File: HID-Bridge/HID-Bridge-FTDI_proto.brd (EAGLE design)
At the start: 33 x 20.3 mm, 7 parts, among them U1 FT232RLSSOP

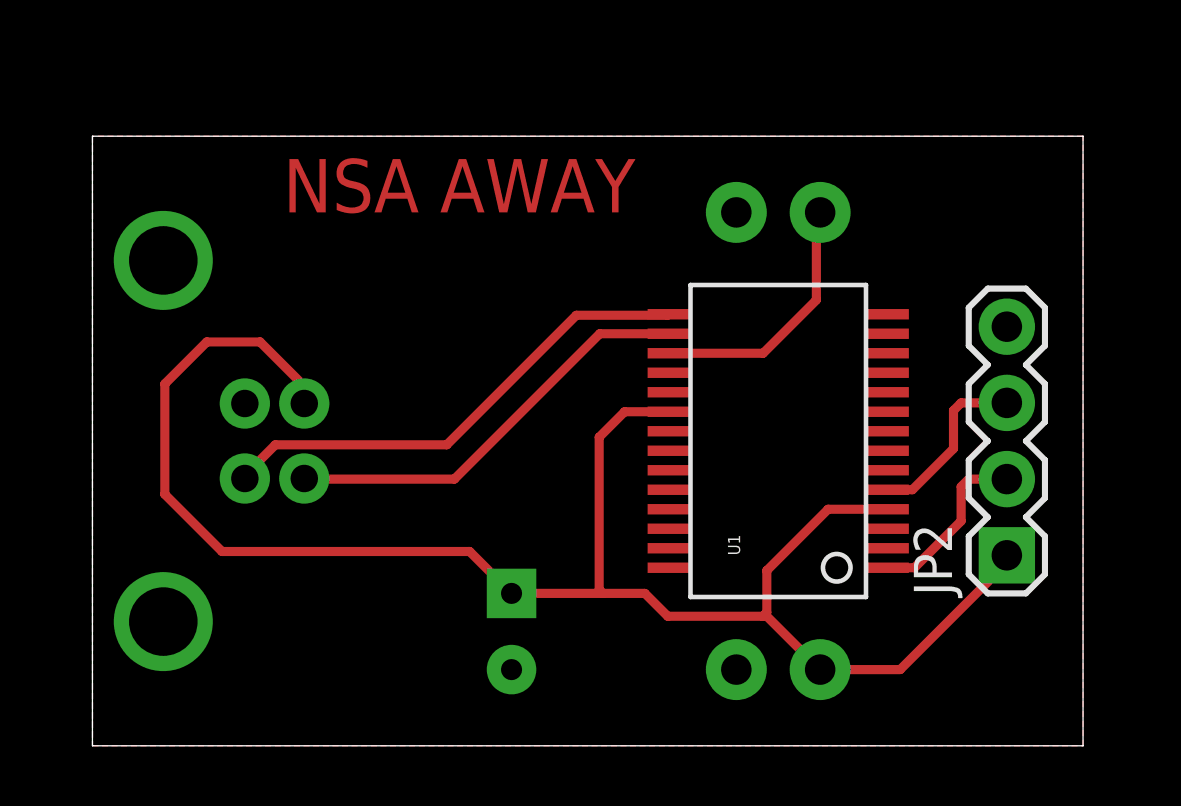
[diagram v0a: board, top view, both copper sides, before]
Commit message: Changes for sides etc.
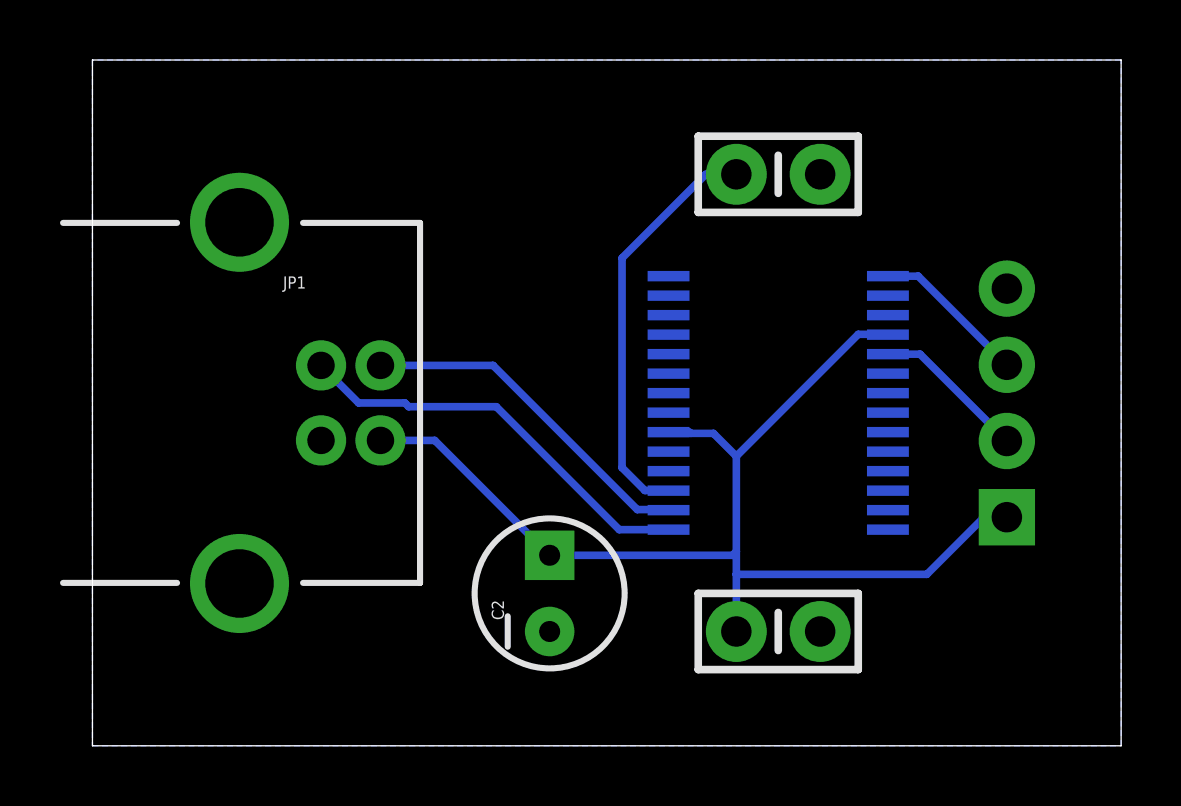
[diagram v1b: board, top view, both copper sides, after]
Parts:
- moved JP1 2.84 mm to (7.62, 11.4), flipped to the top, turned to 0 degrees
- moved C2 1.80 mm to (15.2, 5.08), flipped to the top
- moved JP2 1.27 mm to (30.5, 7.62), flipped to the bottom
- moved C1 1.27 mm to (22.9, 3.81), flipped to the top
- moved C3 1.27 mm to (22.9, 19.1), flipped to the top
- moved U1 1.27 mm to (22.9, 11.4), flipped to the bottom, turned to 270 degrees
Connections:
- net N$1: now also U1.5; no longer U1.1
- net N$4: now also U1.1; no longer U1.5
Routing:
- net 5V: track 56.7 -> 38.5 mm
- net 3.3V: track 8.63 -> 13.8 mm
- net N$2: track 16.5 -> 13.9 mm
- net N$3: track 14.2 -> 11.6 mm
- net N$4: track 5.91 -> 5.19 mm
- net N$1: track 5.86 -> 5.16 mm
- added copper zone on layer 16, net GND
- removed copper zone on layer 1, net GND
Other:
- board size 33 x 20.3 mm -> 34.3 x 22.9 mm
- board text removed: "NSA AWAY"
